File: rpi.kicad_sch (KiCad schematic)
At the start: 1 part, among them J1 26PIN_RPI_HEADER

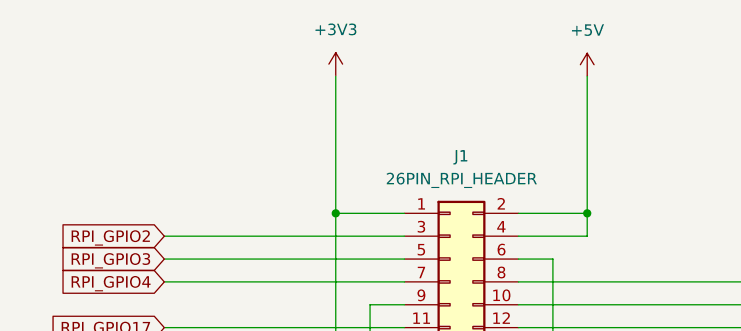
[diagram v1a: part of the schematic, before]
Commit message: after rough draft submission
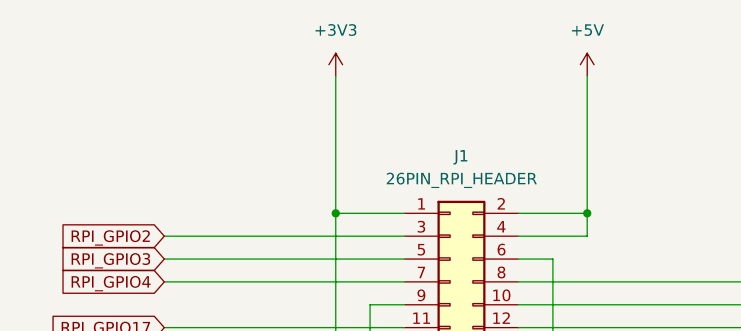
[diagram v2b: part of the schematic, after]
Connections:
- net +3V3: now also J1.1 (Pin_1), J1.17 (Pin_17)
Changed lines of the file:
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@@
 	(symbol
 		(lib_id "power:+3V3")
-		(at 133.35 62.1615 0)
+		(at 133.35 62.23 0)
 		(unit 1)
 		(exclude_from_sim no)
@@
 		(fields_autoplaced yes)
 		(property "Reference" "#PWR041"
-			(at 133.35 65.9715 0)
+			(at 133.35 66.04 0)
 			(effects
 				(font
@@
 		)
 		(property "Value" "+3V3"
-			(at 133.35 57.0815 0)
+			(at 133.35 57.15 0)
 			(effects
 				(font
@@
 		)
 		(property "Footprint" ""
-			(at 133.35 62.1615 0)
+			(at 133.35 62.23 0)
 			(effects
 				(font
@@
 		)
 		(property "Datasheet" ""
-			(at 133.35 62.1615 0)
+			(at 133.35 62.23 0)
 			(effects
 				(font
@@
 		)
 		(property "Description" "Power symbol creates a global label with name \"+3V3\""
-			(at 133.35 62.1615 0)
+			(at 133.35 62.23 0)
 			(effects
 				(font
